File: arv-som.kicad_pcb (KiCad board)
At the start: 2 copper layers, 55 x 40 mm, 11 parts, among them J3 DF40C-100DP-0.4V(51), J4 DF40C-100DP-0.4V(51), U1 MT53D1024M32D4DT-053, U10 TDA19988BHN_C1,557, U11 KSZ9031RNXCA, U13 VIC7100, U3 MT53D1024M32D4DT-053, U8 TPS65086100, U9 GD25LQ256DWIGR

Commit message: Update libraries
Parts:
- J3, J4: footprint antmicro-footprints:HRS_DF40C-100DP-0.4V(51) -> arv-som-footprints:HRS_DF40C-100DP-0.4V(51)
- N1: footprint antmicro-footprints:antmicro-logo_scaled_12mm -> arv-som-footprints:antmicro-logo_scaled_12mm
- N2: footprint antmicro-footprints:oshw-logo -> arv-som-footprints:oshw-logo
- U1, U3: footprint antmicro-footprints:BGA-200_10.0x14.5mm_Layout12x22_P0.80x0.65mm -> arv-som-footprints:BGA-200_10.0x14.5mm_Layout12x22_P0.80x0.65mm
- U10: footprint antmicro-footprints:QFN50P900X900X100-65N -> arv-som-footprints:QFN50P900X900X100-65N
- U11: footprint antmicro-footprints:QFN-48-Microchip-QFN77-48LD-PL-2 -> arv-som-footprints:QFN-48-Microchip-QFN77-48LD-PL-2
- U13: footprint antmicro-footprints:vic7100 -> arv-som-footprints:vic7100
- U8: footprint antmicro-footprints:QFN50P900X900X80-65N -> arv-som-footprints:QFN50P900X900X80-65N
- U9: footprint antmicro-footprints:8-WSON-6x5 -> arv-som-footprints:8-WSON-6x5
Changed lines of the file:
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@@
     (add_net nRPIBOOT)
   )
-  (module antmicro-footprints:BGA-200_10.0x14.5mm_Layout12x22_P0.80x0.65mm (layer F.Cu)
+  (module arv-som-footprints:BGA-200_10.0x14.5mm_Layout12x22_P0.80x0.65mm (layer F.Cu)
     (at 137.06 74.44 180)
     (descr "BGA-200, 14.5x10.0mm, 200 Ball, 12x22 Layout, 0.8x0.65mm Pitch, http://www.issi.com/WW/pdf/43-46LQ32256A-AL.pdf")
@@
     )
   )
-  (module antmicro-footprints:BGA-200_10.0x14.5mm_Layout12x22_P0.80x0.65mm (layer F.Cu)
+  (module arv-som-footprints:BGA-200_10.0x14.5mm_Layout12x22_P0.80x0.65mm (layer F.Cu)
     (at 175.13 74.51 180)
     (descr "BGA-200, 14.5x10.0mm, 200 Ball, 12x22 Layout, 0.8x0.65mm Pitch, http://www.issi.com/WW/pdf/43-46LQ32256A-AL.pdf")
@@
     )
   )
-  (module antmicro-footprints:oshw-logo (layer F.Cu)
+  (module arv-som-footprints:oshw-logo (layer F.Cu)
     (at 134.02 85.47)
     (attr virtual)
@@
       (xy -1.520547 2.559315)) (layer F.Mask) (width 0.01))
   )
-  (module antmicro-footprints:antmicro-logo_scaled_12mm (layer F.Cu)
+  (module arv-som-footprints:antmicro-logo_scaled_12mm (layer F.Cu)
     (at 143.52 58.47)
     (attr virtual)
@@
     )
   )
-  (module antmicro-footprints:8-WSON-6x5 (layer F.Cu)
+  (module arv-som-footprints:8-WSON-6x5 (layer F.Cu)
     (at 172.520001 90.958002 90)
     (fp_text reference U9 (at 0.5 -1.1 270) (layer F.SilkS)
@@
     )
   )
-  (module antmicro-footprints:vic7100 (layer F.Cu)
+  (module arv-som-footprints:vic7100 (layer F.Cu)
     (at 164.830001 61.240002 270)
     (fp_text reference U13 (at -1.016 1.525) (layer F.SilkS)
@@
     )
   )
-  (module antmicro-footprints:QFN-48-Microchip-QFN77-48LD-PL-2 (layer F.Cu)
+  (module arv-som-footprints:QFN-48-Microchip-QFN77-48LD-PL-2 (layer F.Cu)
     (at 173.440001 60.350002 180)
     (fp_text reference U11 (at -4.9 0 90) (layer F.SilkS)
@@
     )
   )
-  (module antmicro-footprints:QFN50P900X900X100-65N (layer F.Cu)
+  (module arv-som-footprints:QFN50P900X900X100-65N (layer F.Cu)
     (at 145.910001 87.800002 270)
     (fp_text reference U10 (at -5.85 -2.6) (layer F.SilkS)
@@
     )
   )
-  (module antmicro-footprints:QFN50P900X900X80-65N (layer F.Cu)
+  (module arv-som-footprints:QFN50P900X900X80-65N (layer F.Cu)
     (at 163.990001 87.580002 180)
     (fp_text reference U8 (at -5.9 -2.35 90) (layer F.SilkS)
@@
     )
   )
-  (module "antmicro-footprints:HRS_DF40C-100DP-0.4V(51)" (layer B.Cu)
+  (module "arv-som-footprints:HRS_DF40C-100DP-0.4V(51)" (layer B.Cu)
     (at 155.120001 91.970002 180)
     (fp_text reference J4 (at -10.25 -2.5) (layer B.SilkS)
@@
     )
   )
-  (module "antmicro-footprints:HRS_DF40C-100DP-0.4V(51)" (layer B.Cu)
+  (module "arv-som-footprints:HRS_DF40C-100DP-0.4V(51)" (layer B.Cu)
     (at 155.120001 57.970002 180)
     (fp_text reference J3 (at 10 2.5) (layer B.SilkS)

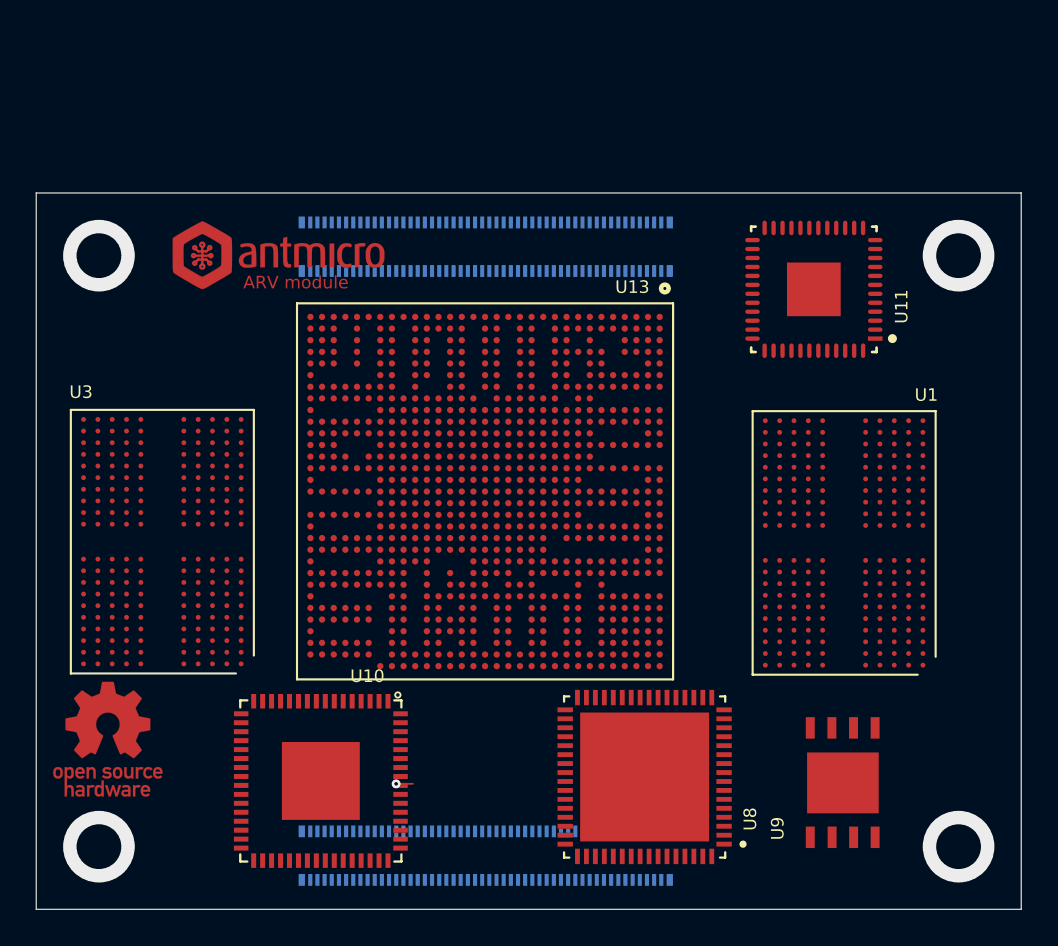
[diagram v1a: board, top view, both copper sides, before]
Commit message: Added DDR layout (wip)
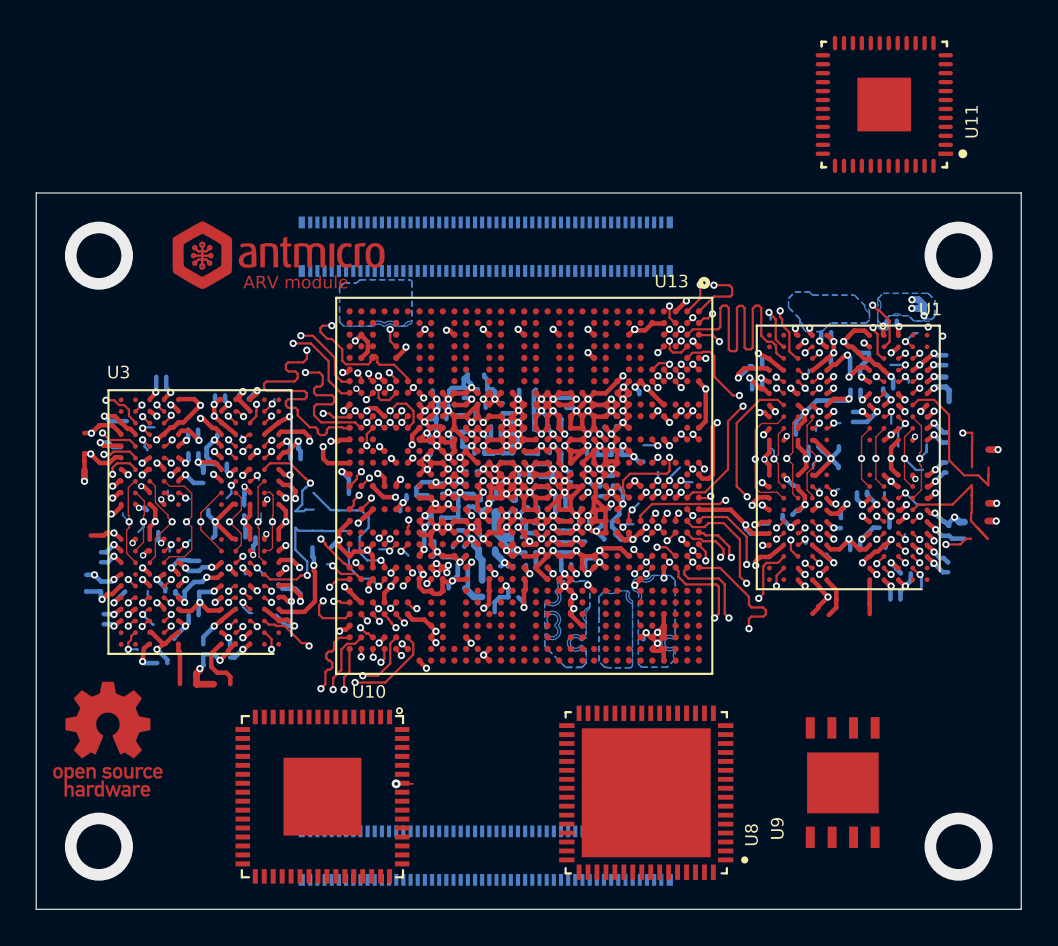
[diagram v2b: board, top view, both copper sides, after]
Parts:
- moved U11 11.0 mm to (177.4, 50.0)
- moved U1 4.78 mm to (175.4, 69.7)
- moved U3 2.37 mm to (139.2, 73.3)
- moved U13 2.21 mm to (167.0, 60.9)
- moved U8 0.88 mm to (164.1, 88.5)
- moved U10 0.88 mm to (146.0, 88.7)
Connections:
- U13 pad AJ5: (no net) -> DDR1_DQ31
- U3 pad AB4: VDD2 -> VDDQ
- U3 pad B10: VDDQ -> VDD2
- U3 pad B8: VDDQ -> VDD2
- U3 pad F5: VDD2 -> VDDQ
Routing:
- net GND: track 0.00 -> 408.6 mm, vias 0 -> 227
- net VCC_1V1: track 0.00 -> 71.9 mm, vias 0 -> 32
- net VCC_0V9: track 0.00 -> 60.5 mm, vias 0 -> 29
- net VDD2: track 0.00 -> 58.6 mm, vias 0 -> 41
- net VDDQ: track 0.00 -> 53.4 mm, vias 0 -> 40
- net VDD1: track 0.00 -> 37.1 mm, vias 0 -> 17
- net DDR1_A03: track 0.00 -> 31.2 mm, vias 0 -> 2
- net DDR1_A02: track 0.00 -> 31.0 mm, vias 0 -> 2
- net DDR1_A00: track 0.00 -> 30.2 mm, vias 0 -> 2
- net DDR1_A05: track 0.00 -> 29.9 mm, vias 0 -> 2
- net DDR1_A01: track 0.00 -> 29.9 mm, vias 0 -> 2
- net DDR0_A04: track 0.00 -> 29.8 mm, vias 0 -> 2
- net DDR1_CS2: track 0.00 -> 29.4 mm, vias 0 -> 2
- net DDR1_A04: track 0.00 -> 28.9 mm, vias 0 -> 2
- net VCC_3V3: track 0.00 -> 28.8 mm, vias 0 -> 7
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- added copper zone on B.Cu, net (none)
- added copper zone on In2.Cu, net (none)
- added copper zone on In4.Cu, net (none)
- added copper zone on In7.Cu, net (none)
- added copper zone on In9.Cu, net (none)
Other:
- copper layers 2 -> 12
